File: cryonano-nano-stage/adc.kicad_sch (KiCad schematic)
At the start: 0 parts

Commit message: preliminary components added
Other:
- added sheet Isolation (isolation.kicad_sch)
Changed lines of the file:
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@@
 	(generator_version "10.0")
 	(paper "A4")
+	(sheet
+		(at 63.5 63.5)
+		(size 12.7 25.4)
+		(exclude_from_sim no)
+		(in_bom no)
+		(on_board no)
+		(dnp yes)
+		(fields_autoplaced yes)
+		(stroke
+			(width 0.1524)
+			(type solid)
+		)
+		(fill
+			(color 0 0 0 0)
+		)
+		(property "Sheetname" "Isolation"
+			(at 63.5 62.7884 0)
+			(show_name no)
+			(do_not_autoplace no)
+			(effects
+				(font
+					(size 1.27 1.27)
+				)
+				(justify left bottom)
+			)
+		)
+		(property "Sheetfile" "isolation.kicad_sch"
+			(at 63.5 89.4846 0)
+			(hide yes)
+			(show_name no)
+			(do_not_autoplace no)
+			(effects
+				(font
+					(size 1.27 1.27)
+				)
+				(justify left top)
+			)
+		)
+		(instances
+			(project "cryonano-nano-stage"
+				(path "/549c6da5-71cb-4d9c-a0a2-c409a6f93509/93ac0006-beae-45e2-a2f0-36893f5b0c34"
+					(page "11")
+				)
+			)
+		)
+	)
 )

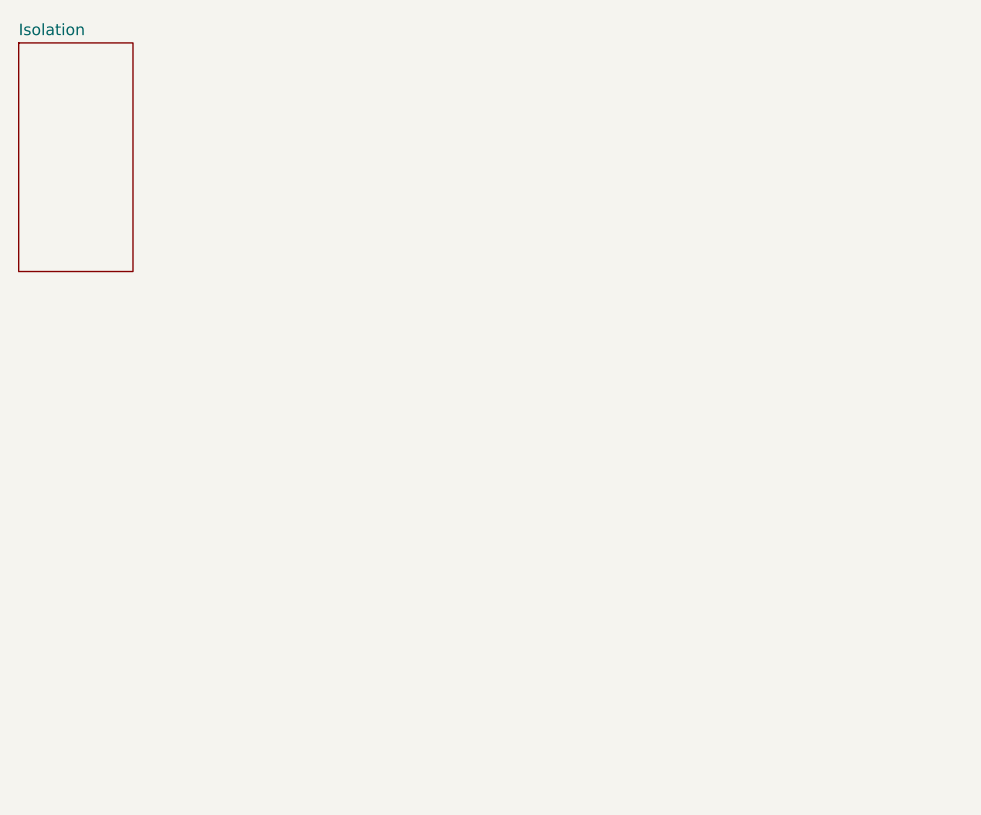
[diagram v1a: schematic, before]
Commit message: sch updated
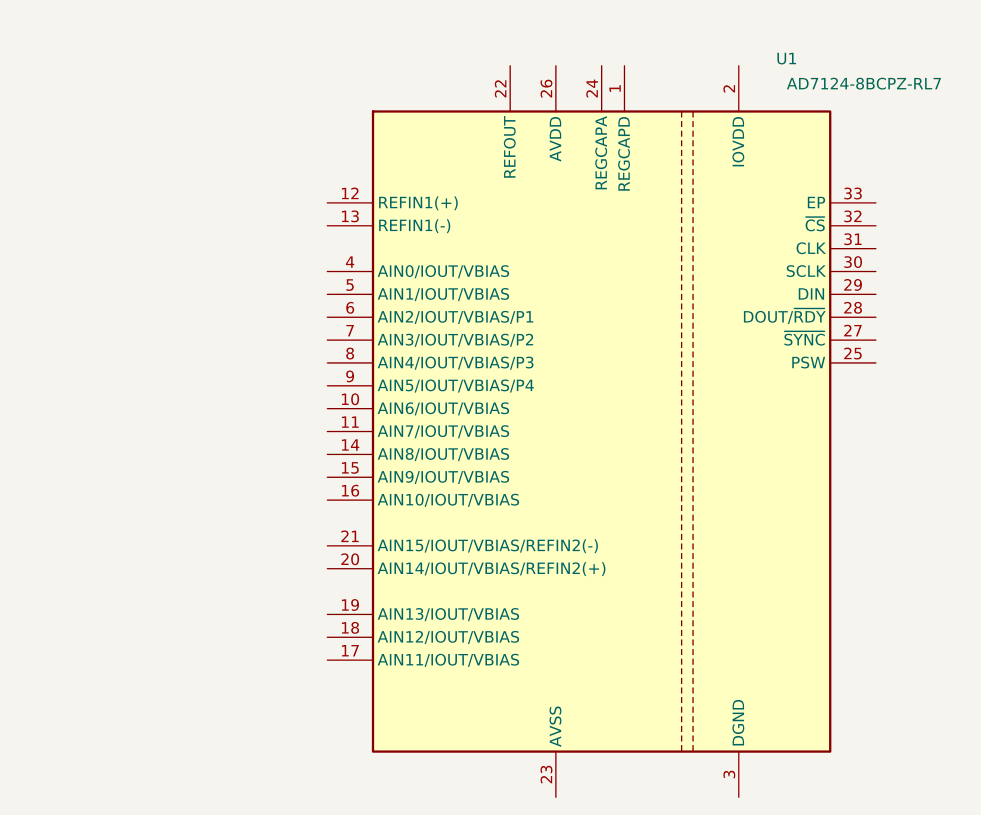
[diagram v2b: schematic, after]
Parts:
- added U1: AD7124-8BCPZ-RL7, QFN50P500X500X80-33N-D, symbol symbols:AD7124-8BCPZ-RL7
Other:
- removed sheet Isolation
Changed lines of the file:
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@@
 	(generator_version "10.0")
 	(paper "A4")
-	(sheet
-		(at 63.5 63.5)
-		(size 12.7 25.4)
-		(exclude_from_sim no)
-		(in_bom no)
-		(on_board no)
-		(dnp yes)
-		(fields_autoplaced yes)
-		(stroke
-			(width 0.1524)
-			(type solid)
-		)
-		(fill
-			(color 0 0 0 0)
-		)
-		(property "Sheetname" "Isolation"
-			(at 63.5 62.7884 0)
-			(show_name no)
-			(do_not_autoplace no)
-			(effects
-				(font
-					(size 1.27 1.27)
-				)
-				(justify left bottom)
-			)
-		)
-		(property "Sheetfile" "isolation.kicad_sch"
-			(at 63.5 89.4846 0)
-			(hide yes)
-			(show_name no)
-			(do_not_autoplace no)
-			(effects
-				(font
-					(size 1.27 1.27)
-				)
-				(justify left top)
-			)
-		)
-		(instances
-			(project "cryonano-nano-stage"
-				(path "/549c6da5-71cb-4d9c-a0a2-c409a6f93509/93ac0006-beae-45e2-a2f0-36893f5b0c34"
-					(page "11")
-				)
-			)
-		)
-	)
-)

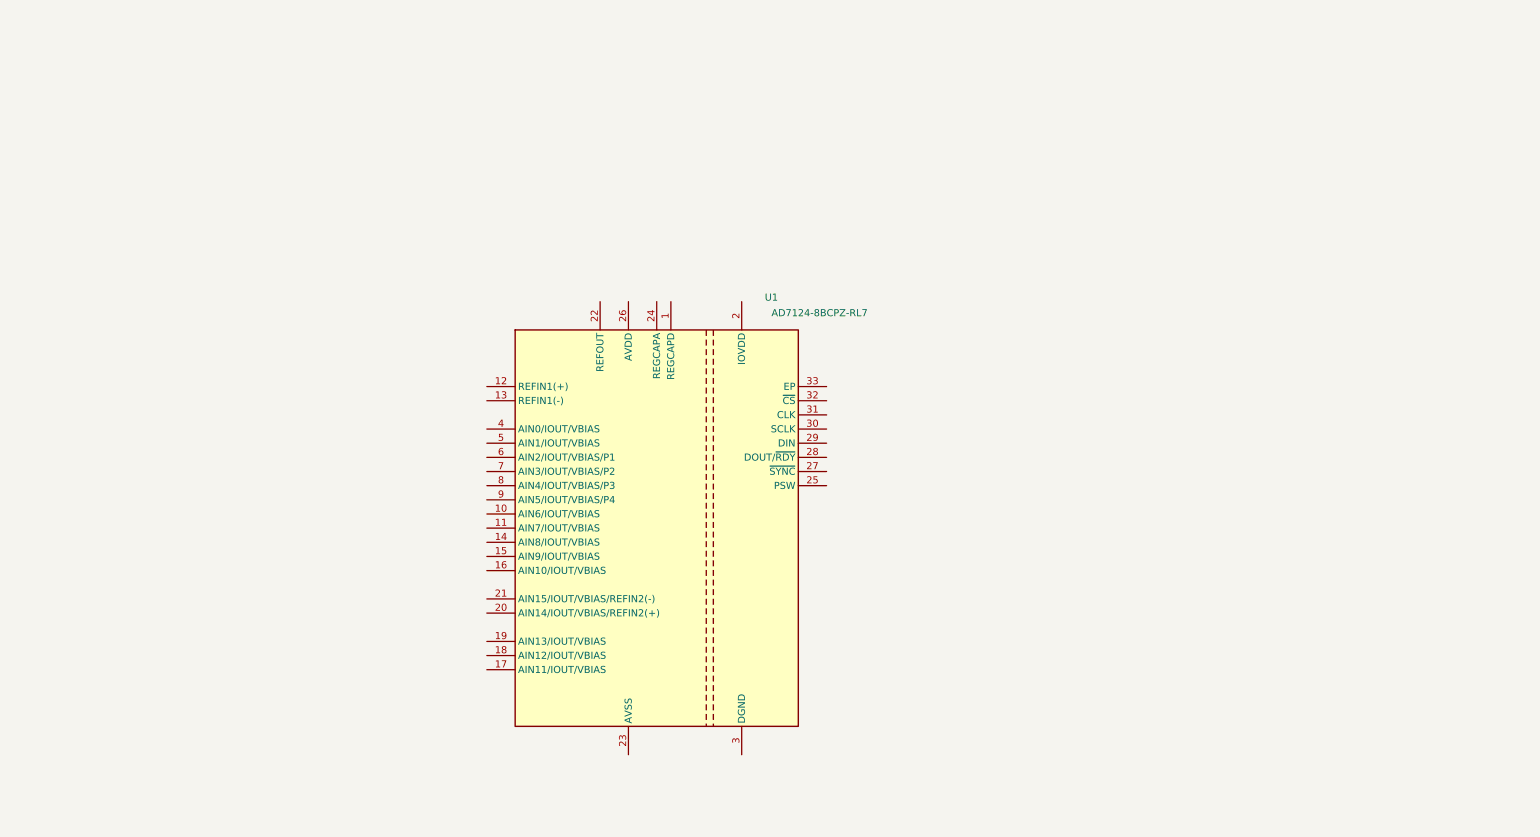
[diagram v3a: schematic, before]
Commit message: sch improved
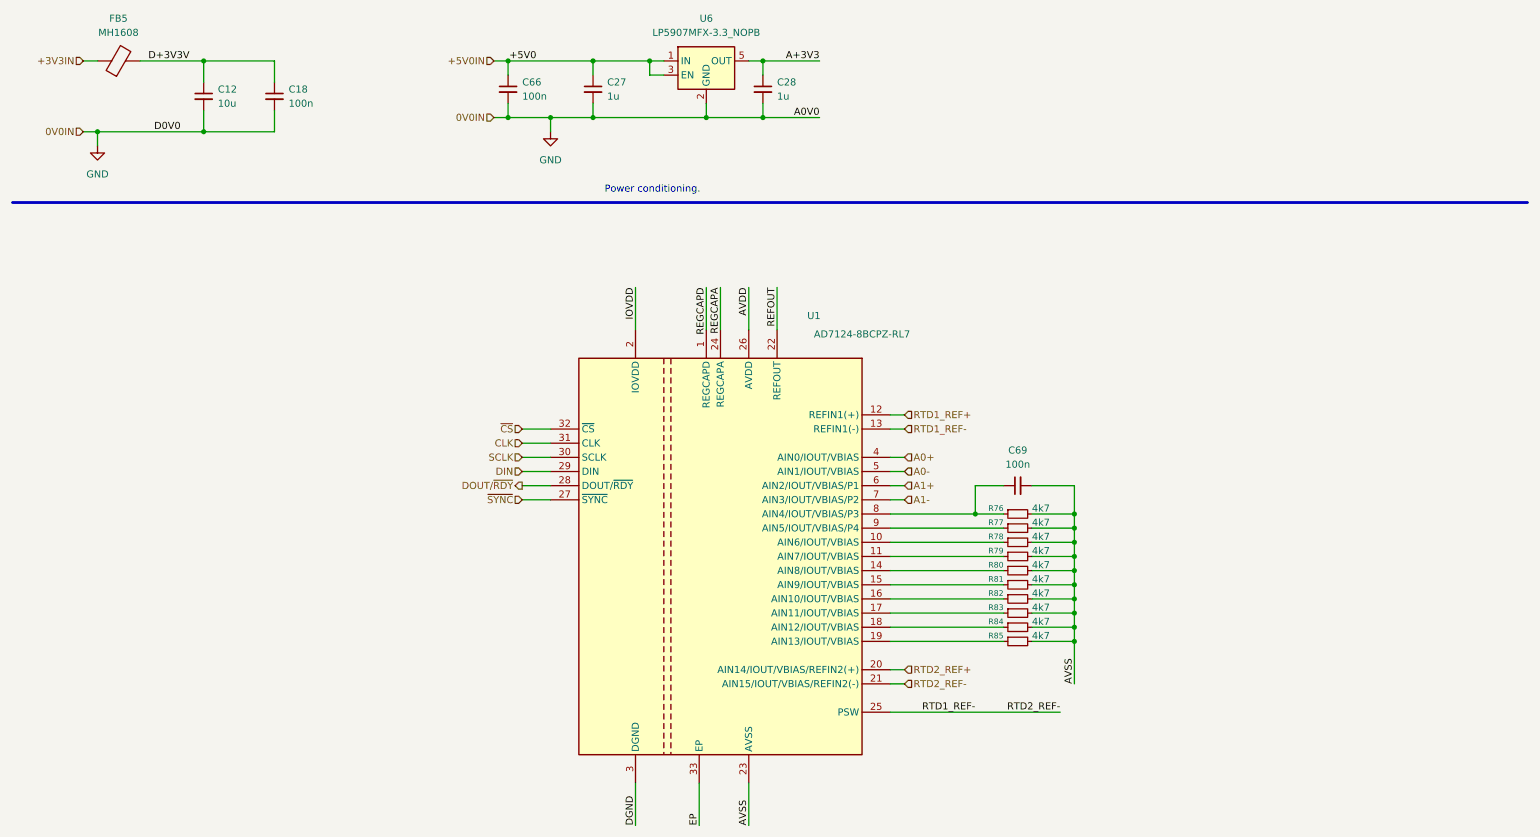
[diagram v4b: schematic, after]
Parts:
- added C12: 10u, Capacitor_SMD:C_0805_2012Metric, symbol Device:C_Small
- added C18, C66, C69: 100n, Capacitor_SMD:C_0603_1608Metric, symbol Device:C_Small
- added C27, C28: 1u, Capacitor_SMD:C_0603_1608Metric, symbol Device:C_Small
- added FB5: MH1608, Inductor_SMD:L_0603_1608Metric, symbol Device:FerriteBead
- added R76, R77, R78, R79, R80, R81, R82, R83, R84, R85: 4k7, Resistor_SMD:R_0603_1608Metric, symbol Device:R_Small
- added U6: LP5907MFX-3.3_NOPB, SOT95P280X145-5N, symbol symbols:LP5907MFX-3.3_NOPB
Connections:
- net REGCAPD: now reaches U1.1 (REGCAPD)
- net at U1.10 (AIN6/IOUT/VBIAS): now also R78.1
- net at U1.11 (AIN7/IOUT/VBIAS): now also R79.1
- net RTD1_REF+: now reaches U1.12 (REFIN1(+))
- net RTD1_REF-: now reaches U1.13 (REFIN1(-))
- net RTD1_REF-: now also U1.21 (AIN15/IOUT/VBIAS/REFIN2(-)), U1.25 (PSW)
- net at U1.14 (AIN8/IOUT/VBIAS): now also R80.1
- net at U1.15 (AIN9/IOUT/VBIAS): now also R81.1
- net at U1.16 (AIN10/IOUT/VBIAS): now also R82.1
- net at U1.17 (AIN11/IOUT/VBIAS): now also R83.1
- net at U1.18 (AIN12/IOUT/VBIAS): now also R84.1
- net at U1.19 (AIN13/IOUT/VBIAS): now also R85.1
- net IOVDD: now reaches U1.2 (IOVDD)
- net RTD2_REF+: now reaches U1.20 (AIN14/IOUT/VBIAS/REFIN2(+))
- net REFOUT: now reaches U1.22 (REFOUT)
- net AVSS: now reaches U1.23 (AVSS)
- net AVSS: now also C69.2, R76.2, R77.2, R78.2, R79.2, R80.2, R81.2, R82.2, R83.2, R84.2, R85.2
- net REGCAPA: now reaches U1.24 (REGCAPA)
- net AVDD: now reaches U1.26 (AVDD)
- net ~{SYNC}: now reaches U1.27 (~{SYNC})
- net DOUT/~{RDY}: now reaches U1.28 (DOUT/~{RDY})
- net DIN: now reaches U1.29 (DIN)
- net DGND: now reaches U1.3 (DGND)
- net SCLK: now reaches U1.30 (SCLK)
- net CLK: now reaches U1.31 (CLK)
- net ~{CS}: now reaches U1.32 (~{CS})
- net EP: now reaches U1.33 (EP)
- net A0+: now reaches U1.4 (AIN0/IOUT/VBIAS)
- net A0-: now reaches U1.5 (AIN1/IOUT/VBIAS)
- net A1+: now reaches U1.6 (AIN2/IOUT/VBIAS/P1)
- net A1-: now reaches U1.7 (AIN3/IOUT/VBIAS/P2)
- net at U1.8 (AIN4/IOUT/VBIAS/P3): now also C69.1, R76.1
- net at U1.9 (AIN5/IOUT/VBIAS/P4): now also R77.1
- new net +3V3IN: FB5.1
- new net +5V0IN: C27.1, C66.1, U6.1 (IN), U6.3 (EN)
- new net A+3V3: C28.1, U6.5 (OUT)
- new net D+3V3V: C12.1, C18.1, FB5.2
- new net GND: C12.2, C18.2, C27.2, C28.2, C66.2, U6.2 (GND)
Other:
- note added: "Power conditioning."
- company: (none) -> Cryonano Labs Pvt. Ltd.
- title: (none) -> Nano stage controller
- moved on the sheet: U1
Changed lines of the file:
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@@
 	(generator_version "10.0")
 	(paper "A4")
+	(title_block
+		(title "Nano stage controller")
+		(date "08-08-2026")
+		(company "Cryonano Labs Pvt. Ltd.")
+		(comment 1 "SBB")
+		(comment 4 "0.0.1")
+		(comment 5 "0.0.1")
+		(comment 6 "08-08-2026")
+		(comment 8 "08-08-2026")
+	)
